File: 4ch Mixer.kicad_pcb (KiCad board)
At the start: 2 copper layers, 42 parts, among them J1 3.5mm_Mono_Jack_With_Switch, J2 3.5mm_Mono_Jack_With_Switch, J3 3.5mm_Mono_Jack_With_Switch, J4 3.5mm_Mono_Jack_With_Switch, J5 3.5mm_Mono_Jack_With_Switch, J6 3.5mm_Mono_Jack_With_Switch, P1 CONN_02X08, U1 TL074, U2 TL072

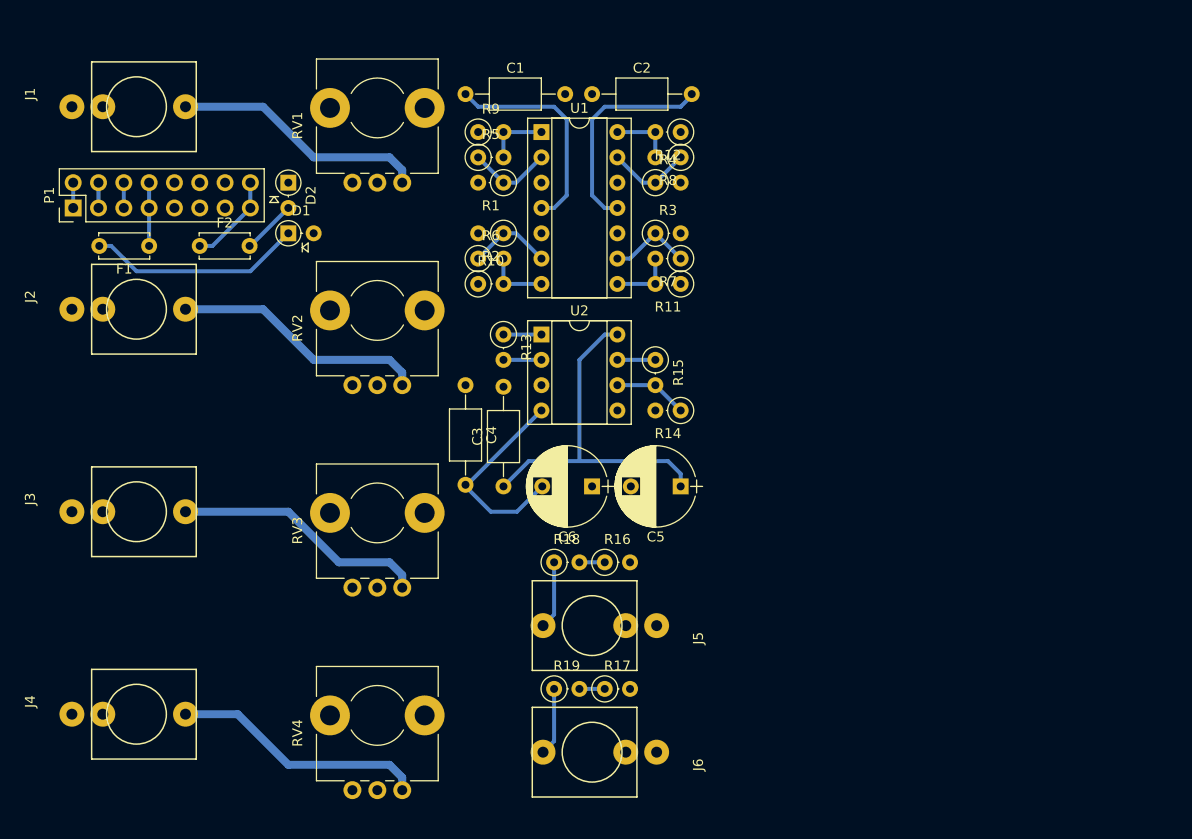
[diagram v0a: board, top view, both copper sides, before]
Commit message: Created PCB.  Need to look over carefully.
Need to measure potentiometer footprint to ensure it is correct.
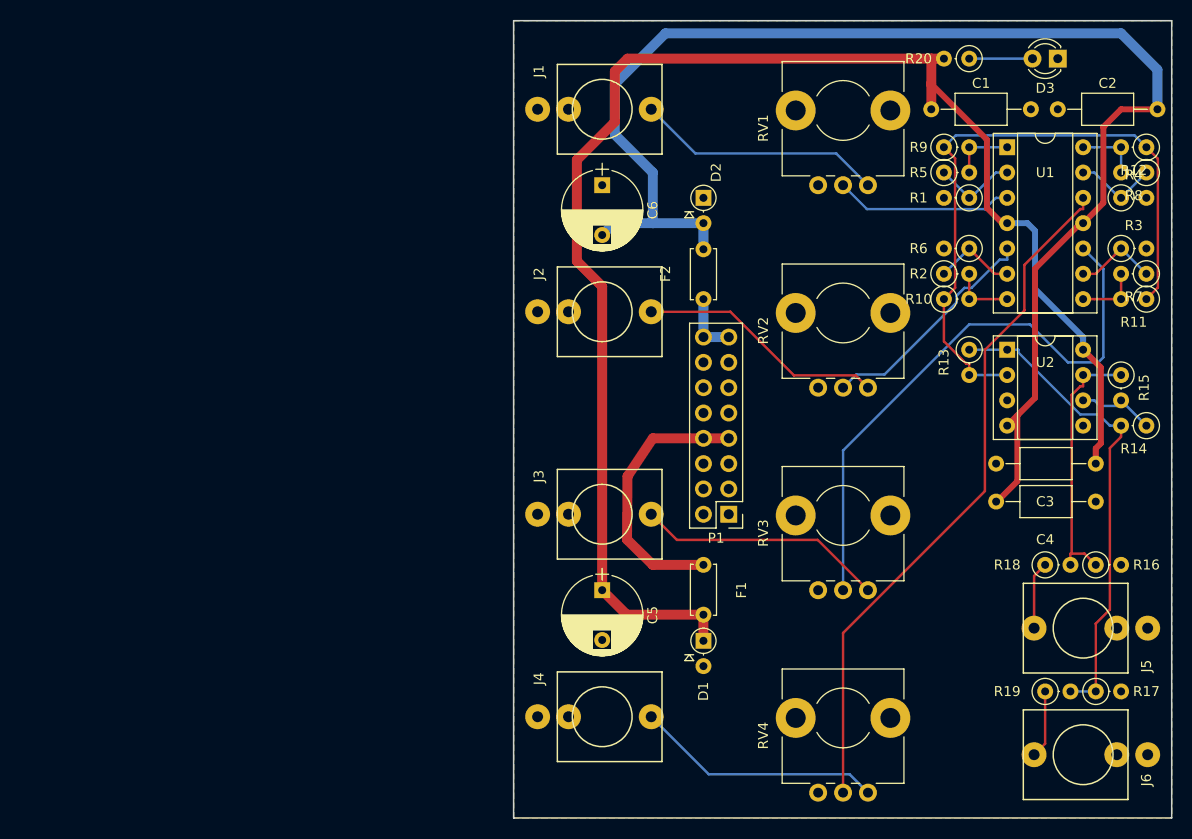
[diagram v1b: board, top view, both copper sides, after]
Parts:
- added D3: LED, LEDs:LED_D3.0mm, F.Cu at (169.9, 54.9)
- added R20: 1k, Resistors_THT:R_Axial_DIN0207_L6.3mm_D2.5mm_P2.54mm_Vertical, F.Cu at (161.0, 54.9)
- moved P1 72.6 mm to (136.9, 100.6), turned to 180 degrees
- moved C4 64.3 mm to (173.7, 99.3), turned to 180 degrees
- moved F1 64.2 mm to (134.4, 105.7), turned to 270 degrees
- moved C3 59.5 mm to (173.7, 95.5), turned to 180 degrees
- moved D1 58.4 mm to (134.4, 113.3), turned to 270 degrees
- moved F2 50.8 mm to (134.4, 79.0), turned to 90 degrees
- moved J5 49.3 mm to (172.5, 112.0)
- moved J6 49.3 mm to (172.5, 124.7)
- moved R18 49.3 mm to (168.7, 105.7)
- moved R19 49.3 mm to (168.7, 118.4)
- moved R16 49.3 mm to (173.7, 105.7)
- moved R17 49.3 mm to (173.7, 118.4)
- moved R15 46.8 mm to (176.3, 86.6)
- moved R3 46.8 mm to (176.3, 73.9)
- moved R4 46.8 mm to (176.3, 68.8)
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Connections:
- P1 pad 2: Net-(P1-Pad1) -> Net-(P1-Pad2)
- P1 pad 4: Net-(P1-Pad3) -> Net-(P1-Pad4)
- P1 pad 6: Net-(P1-Pad5) -> Net-(P1-Pad6)
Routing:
- net -12VA: track 48.0 -> 141.7 mm
- net +12VA: track 79.1 -> 154.0 mm
- net Net-(RV4-Pad2): track 0.00 -> 69.8 mm
- net Net-(R10-Pad1): track 3.81 -> 66.3 mm
- net Net-(RV3-Pad2): track 0.00 -> 58.9 mm
- net Net-(R13-Pad1): track 6.35 -> 48.8 mm
- net Net-(RV2-Pad2): track 0.00 -> 23.3 mm
- net Net-(F1-Pad1): track 6.35 -> 27.3 mm
- net Net-(R15-Pad1): track 6.35 -> 26.5 mm
- net Net-(RV1-Pad2): track 0.00 -> 17.9 mm
- net Net-(D3-Pad2): track 0.00 -> 6.35 mm
- net Net-(F2-Pad1): track 9.20 -> 6.35 mm
- net Net-(P1-Pad5): track 2.54 -> 0.00 mm
- net Net-(P1-Pad3): track 2.54 -> 0.00 mm
- net Net-(P1-Pad1): track 2.54 -> 0.00 mm
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- added copper zone on B.Cu, net GNDA
- added copper zone on F.Cu, net GNDA
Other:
- board outline added: 66 x 80 mm
